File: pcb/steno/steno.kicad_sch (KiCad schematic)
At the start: 53 parts, among them J1 Conn_01x04, K1 diode-choc, K10 diode-choc, K11 diode-choc, K12 diode-choc, K13 diode-choc, K14 diode-choc, K15 diode-choc, K16 diode-choc, K17 diode-choc, K18 diode-choc, K19 diode-choc, K2 diode-choc, K20 diode-choc, K21 diode-choc, K22 diode-choc, K23 diode-choc, K24 diode-choc, K25 diode-choc, K26 diode-choc, K27 diode-choc, K28 diode-choc, K29 diode-choc, K3 diode-choc, K30 diode-choc, K4 diode-choc, K5 diode-choc, K6 diode-choc, K7 diode-choc, K8 diode-choc, K9 diode-choc, Q1 AO3401A, SW2 SW_Push, U1 MT25QL128ABA1ESE, U2 LCD2.2in, U3 Holyiot_18010_no_underside

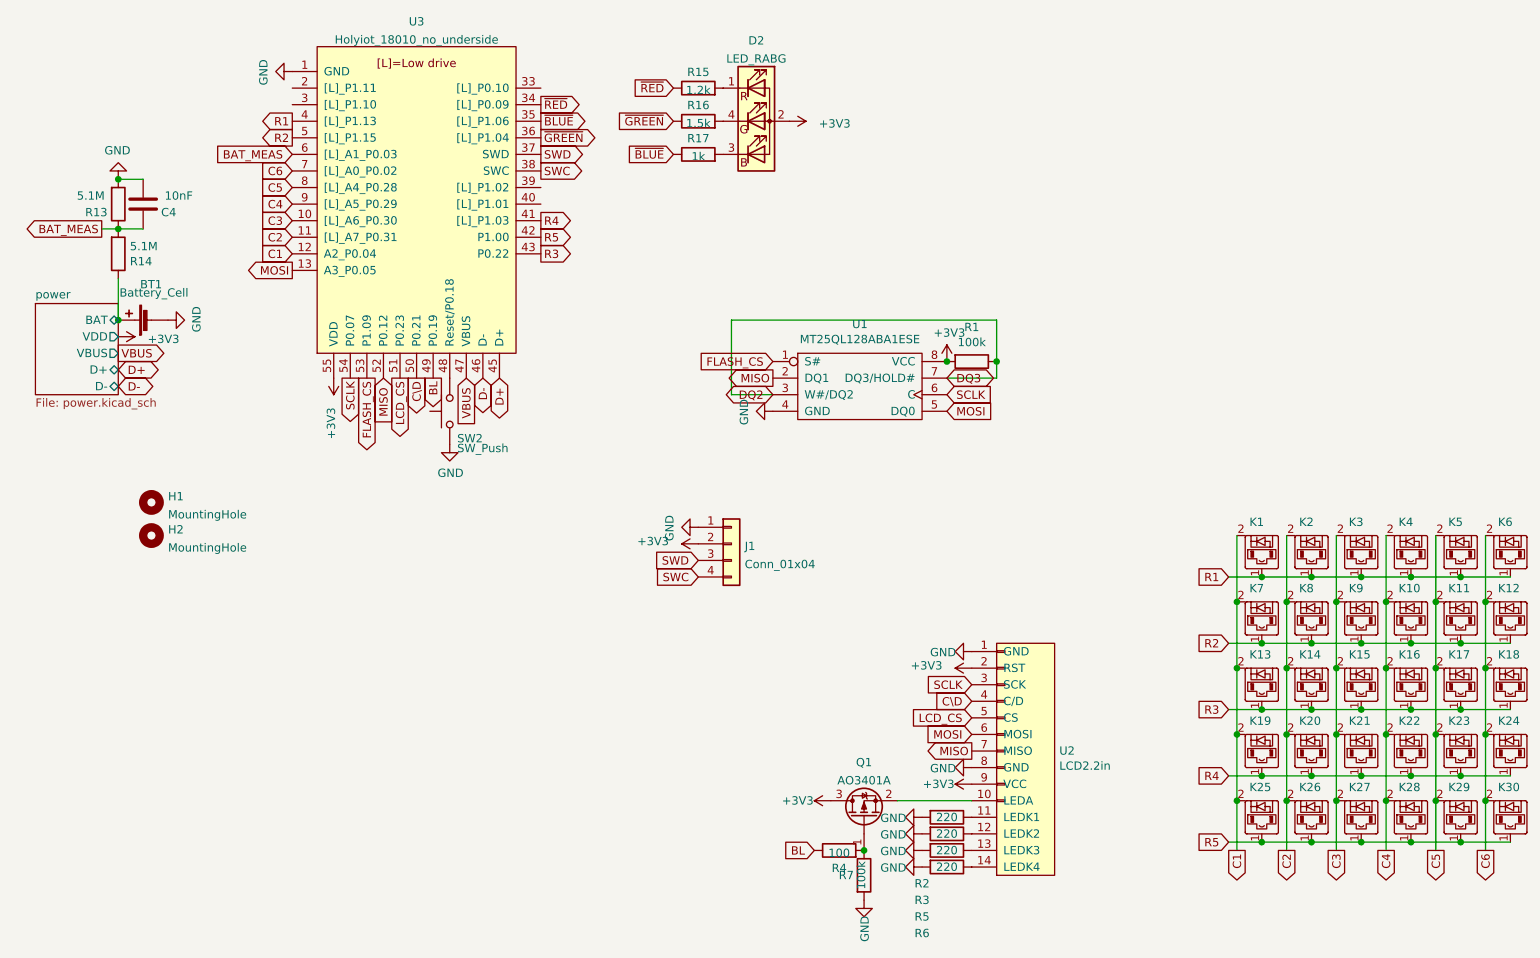
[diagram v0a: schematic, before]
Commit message: [pcb] Auklet 3
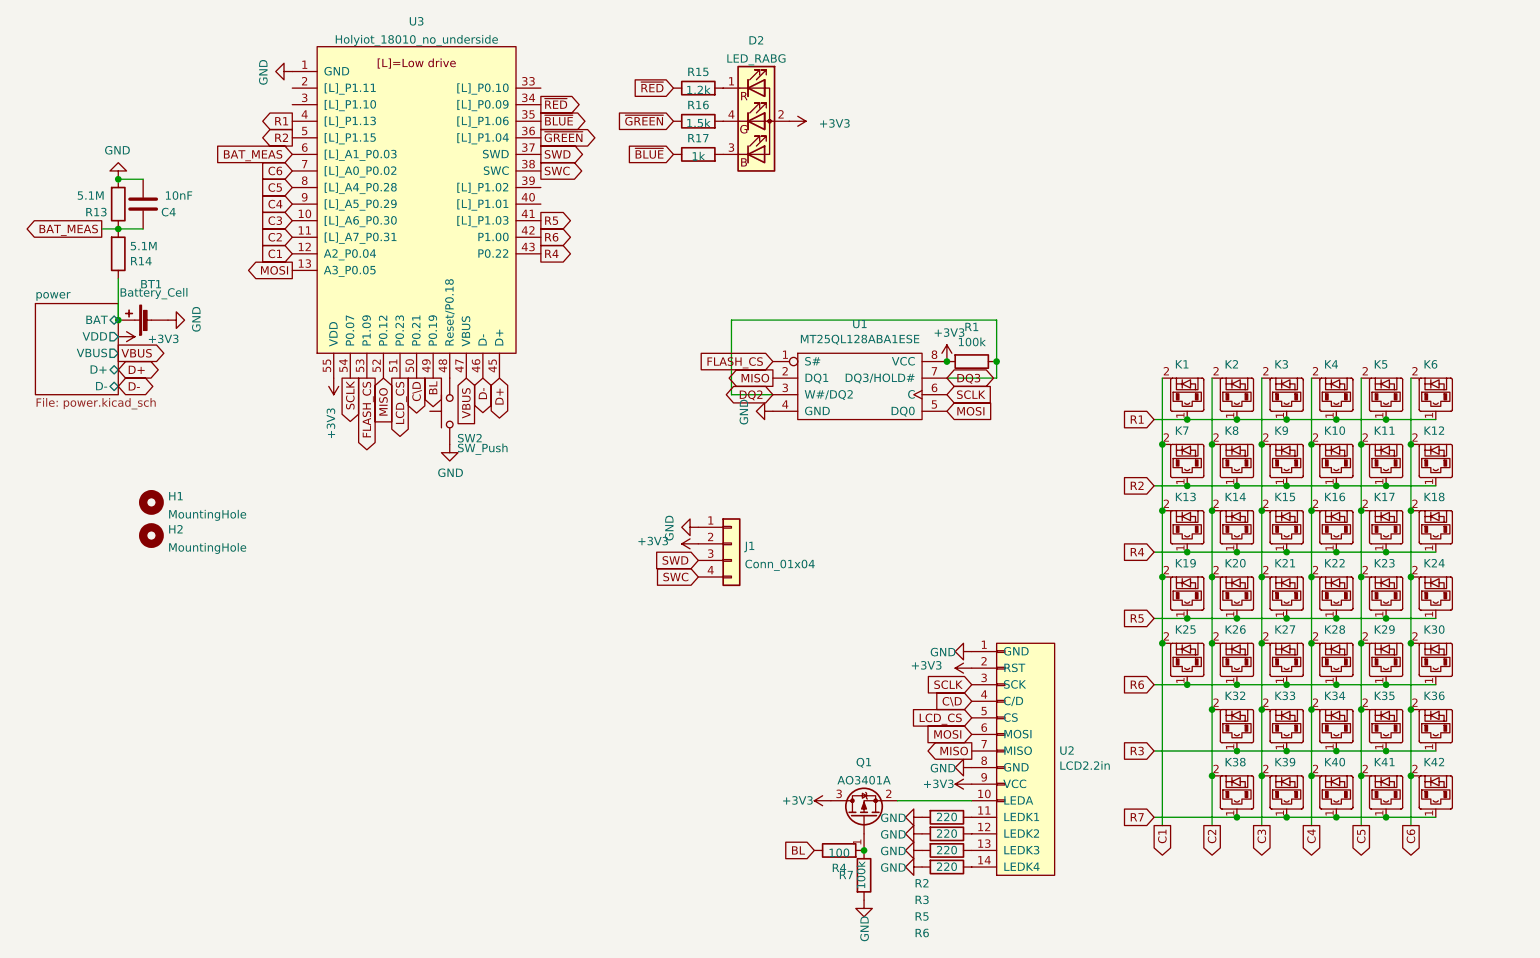
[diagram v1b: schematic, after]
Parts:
- added K32, K33, K34, K35, K36, K38, K39, K40, K41, K42: diode-choc, pg1350:pg1350-D, symbol diode-choc:diode-choc
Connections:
- net C2: now also K32.2, K38.2
- net C3: now also K33.2, K39.2
- net C4: now also K34.2, K40.2
- net C5: now also K35.2, K41.2
- net C6: now also K36.2, K42.2
- net R3: now also K32.1, K33.1, K34.1, K35.1, K36.1; no longer K13.1, K14.1, K15.1, K16.1, K17.1, K18.1, U3.43 (P0.22)
- net R4: now also K13.1, K14.1, K15.1, K16.1, K17.1, K18.1, U3.43 (P0.22); no longer K19.1, K20.1, K21.1, K22.1, K23.1, K24.1, U3.41 ([L]_P1.03)
- net R5: now also K19.1, K20.1, K21.1, K22.1, K23.1, K24.1, U3.41 ([L]_P1.03); no longer K25.1, K26.1, K27.1, K28.1, K29.1, K30.1, U3.42 (P1.00)
- new net R6: K25.1, K26.1, K27.1, K28.1, K29.1, K30.1, U3.42 (P1.00)
- new net R7: K38.1, K39.1, K40.1, K41.1, K42.1
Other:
- moved on the sheet: K1, K10, K11, K12, K13, K14, K15, K16, K17, K18, K19, K2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
